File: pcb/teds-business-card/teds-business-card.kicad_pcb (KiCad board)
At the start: 2 copper layers, 85 x 54 mm, 5 parts, among them U1 NT3H2111W0FHKH

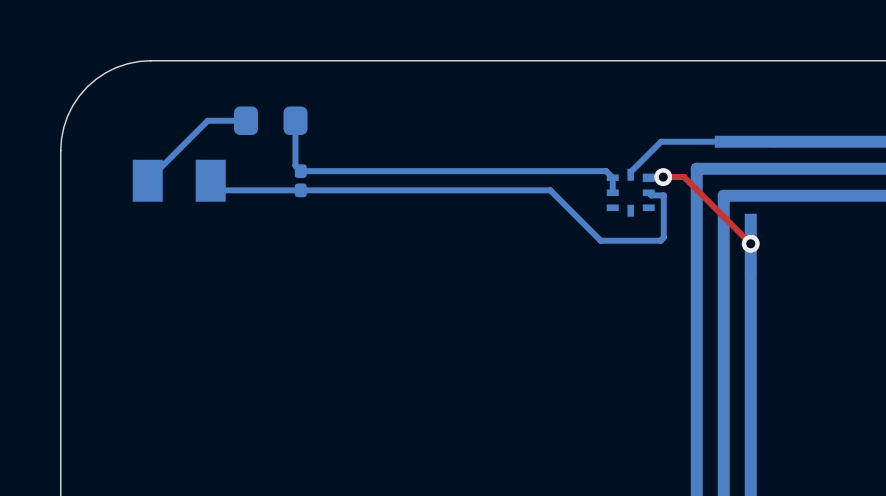
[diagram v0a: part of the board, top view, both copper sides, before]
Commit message: add prod files
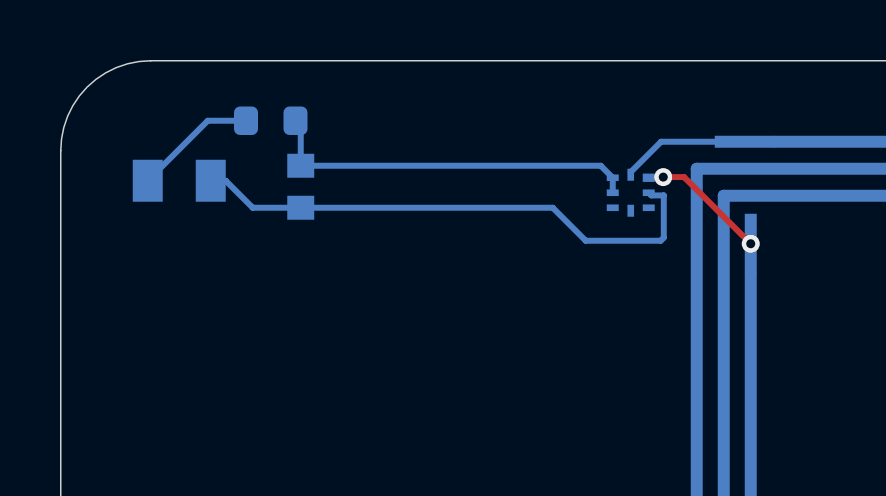
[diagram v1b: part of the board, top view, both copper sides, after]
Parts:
- C1: footprint Capacitor_SMD:C_0201_0603Metric -> easyeda2kicad:C0603
- moved C1 0.20 mm to (128.0, 74.2)
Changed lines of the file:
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@@
 			)
 		)
+		(property "LCSC Part" "C23182"
+			(at 0 0 0)
+			(unlocked yes)
+			(layer "B.Fab")
+			(hide yes)
+			(effects
+				(font
+					(size 1 1)
+					(thickness 0.15)
+				)
+				(justify mirror)
+			)
+		)
 		(property ki_fp_filters "R_*")
 		(sheetname "/")
@@
 		)
 	)
-	(footprint "Capacitor_SMD:C_0201_0603Metric"
+	(footprint "easyeda2kicad:C0603"
 		(layer "B.Cu")
-		(at 128 74 90)
-		(descr "Capacitor SMD 0201 (0603 Metric), square (rectangular) end terminal, IPC-7351 nominal, (Body size source: https://www.vishay.com/docs/20052/crcw0201e3.pdf), generated with kicad-footprint-generator")
-		(tags "capacitor")
+		(at 128 74.2 90)
+		(descr "220nF (224) ±10% 25V")
 		(property "Reference" "C1"
-			(at 0 1.05 90)
+			(at 0 4 270)
 			(layer "B.SilkS")
-			(hide yes)
 			(effects
 				(font
@@
 		)
 		(property "Value" "220nF"
-			(at 0 -1.05 90)
+			(at 0 -4 270)
 			(layer "B.Fab")
-			(hide yes)
 			(effects
 				(font
@@
 		)
 		(property "Datasheet" "~"
-			(at 0 0 90)
+			(at 0 0 270)
 			(layer "B.Fab")
 			(hide yes)
@@
 		)
 		(property "Description" "Unpolarized capacitor"
-			(at 0 0 90)
+			(at 0 0 270)
+			(layer "B.Fab")
+			(hide yes)
+			(effects
+				(font
+					(size 1.27 1.27)
+					(thickness 0.15)
+				)
+				(justify mirror)
+			)
+		)
+		(property "LCSC Part" "C21120"
+			(at 0 0 270)
 			(layer "B.Fab")
 			(hide yes)
@@
 		(sheetfile "teds-business-card.kicad_sch")
 		(attr smd)
-		(fp_line
-			(start 0.7 -0.35)
-			(end -0.7 -0.35)
+		(fp_circle
+			(center -0.8 -0.4)
+			(end -0.77 -0.4)
 			(stroke
-				(width 0.05)
+				(width 0.06)
 				(type solid)
 			)
-			(layer "B.CrtYd")
+			(fill no)
+			(layer "B.SilkS")
 		)
 		(fp_line
-			(start -0.7 -0.35)
-			(end -0.7 0.35)
+			(start 0.8 -0.4)
+			(end -0.8 -0.4)
 			(stroke
 				(width 0.05)
@@
 		)
 		(fp_line
-			(start 0.7 0.35)
-			(end 0.7 -0.35)
+			(start -0.8 -0.4)
+			(end -0.8 0.4)
 			(stroke
 				(width 0.05)
@@
 		)
 		(fp_line
-			(start -0.7 0.35)
-			(end 0.7 0.35)
+			(start 0.8 0.4)
+			(end 0.8 -0.4)
 			(stroke
 				(width 0.05)
@@
 		)
 		(fp_line
-			(start 0.3 -0.15)
-			(end -0.3 -0.15)
-			(stroke
-				(width 0.1)
-				(type solid)
-			)
-			(layer "B.Fab")
-		)
-		(fp_line
-			(start -0.3 -0.15)
-			(end -0.3 0.15)
-			(stroke
-				(width 0.1)
-				(type solid)
-			)
-			(layer "B.Fab")
-		)
-		(fp_line
-			(start 0.3 0.15)
-			(end 0.3 -0.15)
-			(stroke
-				(width 0.1)
-				(type solid)
-			)
-			(layer "B.Fab")
-		)
-		(fp_line
-			(start -0.3 0.15)
-			(end 0.3 0.15)
+			(start -0.8 0.4)
+			(end 0.8 0.4)
 			(stroke
-				(width 0.1)
+				(width 0.05)
 				(type solid)
 			)
-			(layer "B.Fab")
+			(layer "B.CrtYd")
 		)
 		(fp_text user "${REFERENCE}"
-			(at 0 0.68 90)
+			(at 0 0 270)
 			(layer "B.Fab")
 			(effects
 				(font
-					(size 0.25 0.25)
-					(thickness 0.04)
+					(size 1 1)
+					(thickness 0.15)
 				)
 				(justify mirror)
 			)
 		)
-		(pad "" smd roundrect
-			(at -0.345 0 90)
-			(size 0.318 0.36)
-			(layers "B.Paste")
-			(roundrect_rratio 0.25)
-		)
-		(pad "" smd roundrect
-			(at 0.345 0 90)
-			(size 0.318 0.36)
-			(layers "B.Paste")
-			(roundrect_rratio 0.25)
-		)
-		(pad "1" smd roundrect
-			(at -0.32 0 90)
-			(size 0.46 0.4)
-			(layers "B.Cu" "B.Mask")
-			(roundrect_rratio 0.25)
+		(pad "1" smd rect
+			(at -0.7 0 90)
+			(size 0.8 0.9)
+			(layers "B.Cu" "B.Mask" "B.Paste")
 			(net 2 "Net-(LED1-K)")
 			(pintype "passive")
 		)
-		(pad "2" smd roundrect
-			(at 0.32 0 90)
-			(size 0.46 0.4)
-			(layers "B.Cu" "B.Mask")
-			(roundrect_rratio 0.25)
+		(pad "2" smd rect
+			(at 0.7 0 90)
+			(size 0.8 0.9)
+			(layers "B.Cu" "B.Mask" "B.Paste")
 			(net 1 "Net-(U1-VCC)")
 			(pintype "passive")
 		)
 		(embedded_fonts no)
-		(model "${KICAD9_3DMODEL_DIR}/Capacitor_SMD.3dshapes/C_0201_0603Metric.step"
+		(model "${KIPRJMOD}/teds-business-card/libs/easyeda2kicad.3dshapes/C0603_L1.6-W0.8-H0.8.wrl"
 			(offset
 				(xyz 0 0 0)
@@
 		(sheetfile "teds-business-card.kicad_sch")
 		(attr smd)
-		(fp_line
-			(start 1 1)
-			(end 1 0.86)
-			(stroke
-				(width 0.25)
-				(type solid)
-			)
-			(layer "B.SilkS")
-		)
-		(fp_line
-			(start 1 -0.86)
-			(end 1 -1)
-			(stroke
-				(width 0.25)
-				(type solid)
-			)
-			(layer "B.SilkS")
-		)
-		(fp_line
-			(start 1 -1)
-			(end 0.33 -1)
-			(stroke
-				(width 0.25)
-				(type solid)
-			)
-			(layer "B.SilkS")
-		)
-		(fp_line
-			(start 0.33 1)
-			(end 1 1)
-			(stroke
-				(width 0.25)
-				(type solid)
-			)
-			(layer "B.SilkS")
-		)
-		(fp_line
-			(start -0.32 -1)
-			(end -1 -1)
-			(stroke
-				(width 0.25)
-				(type solid)
-			)
-			(layer "B.SilkS")
-		)
-		(fp_line
-			(start -1 1)
-			(end -0.32 1)
-			(stroke
-				(width 0.25)
-				(type solid)
-			)
-			(layer "B.SilkS")
-		)
-		(fp_line
-			(start -1 0.86)
-			(end -1 1)
-			(stroke
-				(width 0.25)
-				(type solid)
-			)
-			(layer "B.SilkS")
-		)
-		(fp_line
-			(start -1 -1)
-			(end -1 -0.86)
-			(stroke
-				(width 0.25)
-				(type solid)
-			)
-			(layer "B.SilkS")
-		)
 		(fp_circle
 			(center -0.8 0.8)
@@
 			)
 		)
-		(property "Description" ""
+		(property "Description" "NFC Square Antenna"
 			(at 0 0 180)
 			(layer "B.Fab")
@@
 	)
 	(segment
-		(start 138.18 73.68)
-		(end 128 73.68)
+		(start 128 73.5)
+		(end 138 73.5)
 		(width 0.2)
 		(layer "B.Cu")
@@
 	)
 	(segment
-		(start 127.825 72)
-		(end 127.825 73.505)
+		(start 128 72.175)
+		(end 127.825 72)
 		(width 0.2)
 		(layer "B.Cu")
@@
 	)
 	(segment
-		(start 138.4 73.9)
-		(end 138.18 73.68)
+		(start 138 73.5)
+		(end 138.4 73.9)
 		(width 0.2)
 		(layer "B.Cu")
@@
 	)
 	(segment
-		(start 127.825 73.505)
-		(end 128 73.68)
+		(start 128 73.5)
+		(end 128 72.175)
 		(width 0.2)
 		(layer "B.Cu")
@@
 	)
 	(segment
-		(start 140.101 75.899)
-		(end 140 76)
+		(start 126.4 74.9)
+		(end 128 74.9)
 		(width 0.2)
 		(layer "B.Cu")
@@
 	)
 	(segment
-		(start 139.6 74.4)
-		(end 139.689 74.489)
+		(start 136.4 74.9)
+		(end 128 74.9)
 		(width 0.2)
 		(layer "B.Cu")
@@
 	)
 	(segment
-		(start 138 76)
-		(end 136.32 74.32)
+		(start 137.5 76)
+		(end 136.4 74.9)
 		(width 0.2)
 		(layer "B.Cu")
@@
 	)
 	(segment
-		(start 139.689 74.489)
-		(end 140.101 74.489)
+		(start 125.32 74.32)
+		(end 125 74)
 		(width 0.2)
 		(layer "B.Cu")
@@
 	)
 	(segment
-		(start 125.32 74.32)
-		(end 125 74)
+		(start 139.6 74.4)
+		(end 139.689 74.489)
 		(width 0.2)
 		(layer "B.Cu")
@@
 	)
 	(segment
-		(start 140 76)
-		(end 138 76)
+		(start 140.101 75.899)
+		(end 140 76)
 		(width 0.2)
 		(layer "B.Cu")
@@
 	)
 	(segment
-		(start 140.101 74.489)
-		(end 140.101 75.899)
+		(start 139.689 74.489)
+		(end 140.101 74.489)
+		(width 0.2)
+		(layer "B.Cu")
+		(net 2)
+	)
+	(segment
+		(start 125.5 74)
+		(end 126.4 74.9)
+		(width 0.2)
+		(layer "B.Cu")
+		(net 2)
+	)
+	(segment
+		(start 125 74)
+		(end 125.5 74)
 		(width 0.2)
 		(layer "B.Cu")
@@
 	)
 	(segment
-		(start 136.32 74.32)
-		(end 128 74.32)
+		(start 140 76)
+		(end 137.5 76)
 		(width 0.2)
 		(layer "B.Cu")
@@
 	)
 	(segment
-		(start 128 74.32)
-		(end 125.32 74.32)
+		(start 140.101 74.489)
+		(end 140.101 75.899)
 		(width 0.2)
 		(layer "B.Cu")
